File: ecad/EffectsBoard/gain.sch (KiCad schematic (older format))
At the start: 6 parts, among them Q1 2N4401BU

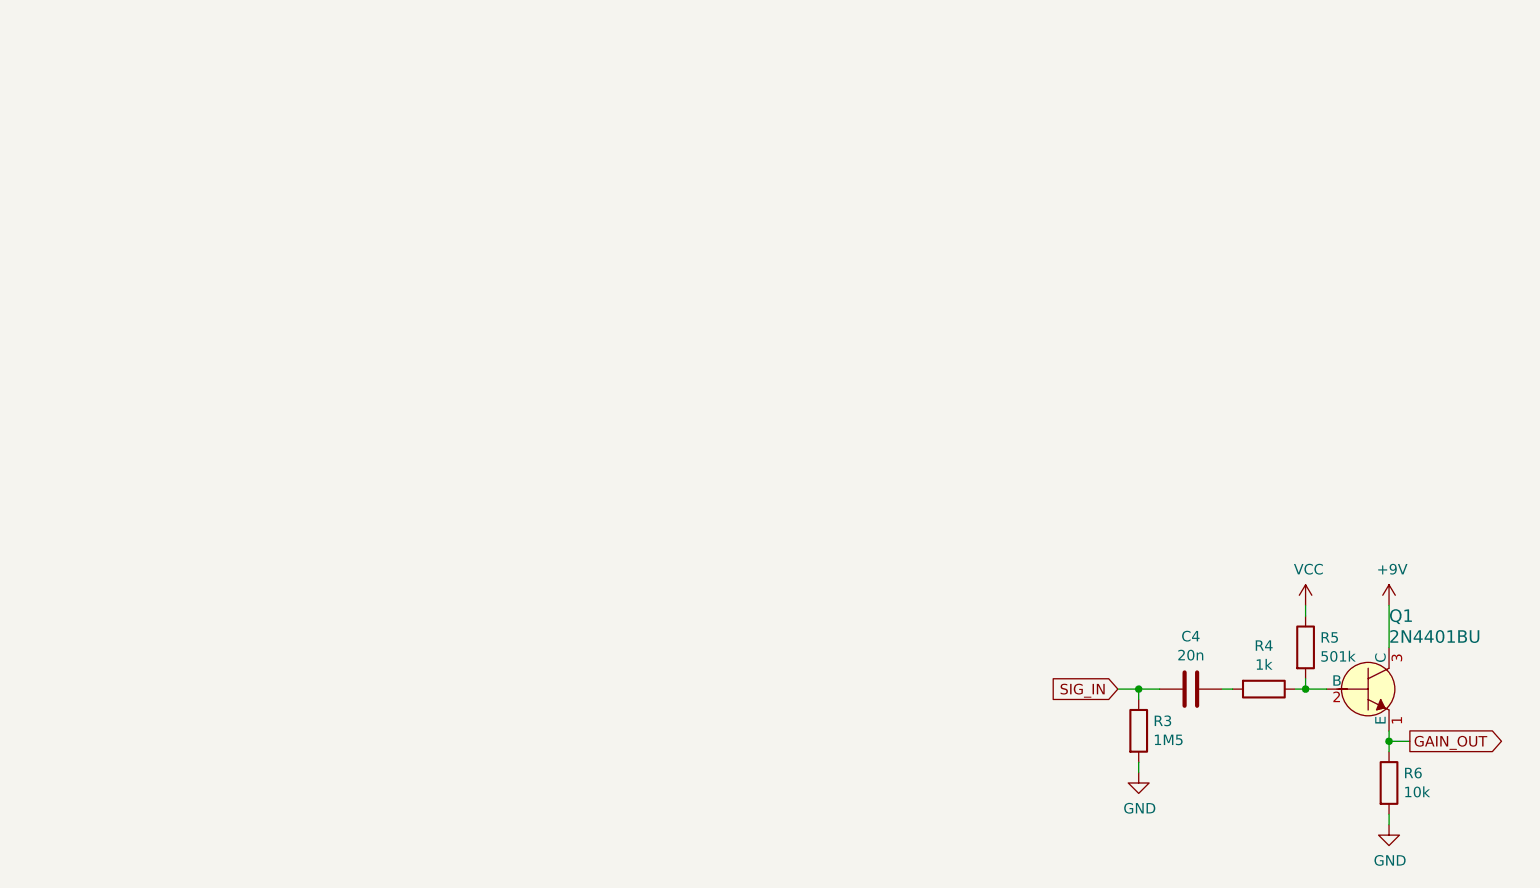
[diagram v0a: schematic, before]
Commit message: Rearrange schematics
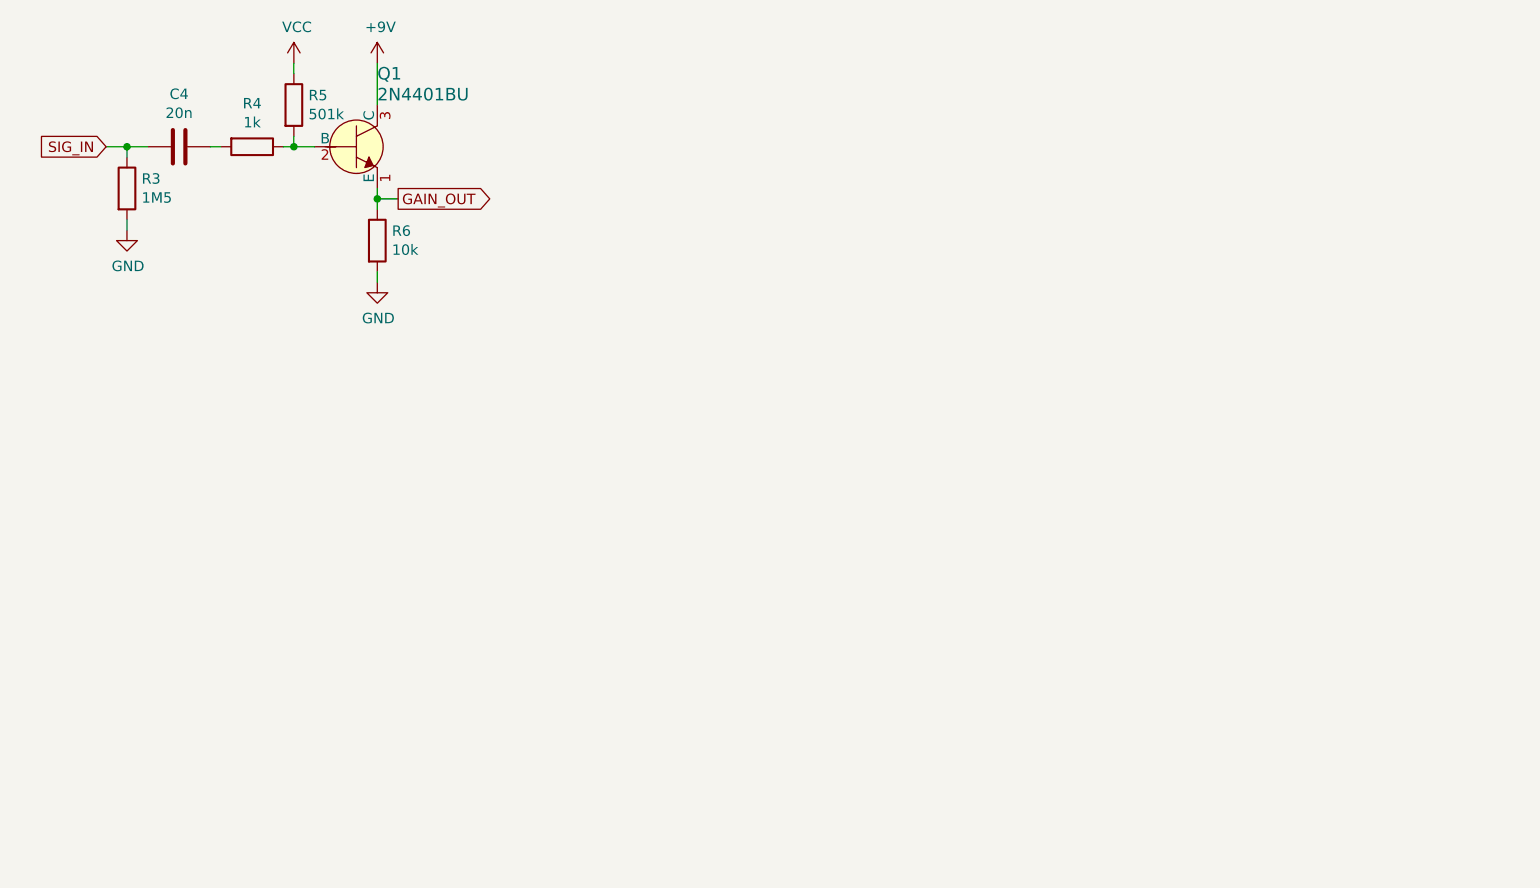
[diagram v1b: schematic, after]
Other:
- moved on the sheet: C4, Q1, R3, R4, R5, R6
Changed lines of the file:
@@
 L Device:R R?
 U 1 1 6030F08B
-P 5750 3900
+P 900 1300
 AR Path="/6030F08B" Ref="R?"  Part="1"
 AR Path="/60306390/6030F08B" Ref="R3"  Part="1"
-F 0 "R3" H 5820 3946 50  0000 L CNN
-F 1 "1M5" H 5820 3855 50  0000 L CNN
-F 2 "" V 5680 3900 50  0001 C CNN
-F 3 "~" H 5750 3900 50  0001 C CNN
-	1    5750 3900
+F 0 "R3" H 970 1346 50  0000 L CNN
+F 1 "1M5" H 970 1255 50  0000 L CNN
+F 2 "" V 830 1300 50  0001 C CNN
+F 3 "~" H 900 1300 50  0001 C CNN
+	1    900  1300
 	1    0    0    -1
 $EndComp
@@
 L power:GND #PWR?
 U 1 1 6030F091
-P 5750 4100
+P 900 1500
 AR Path="/6030F091" Ref="#PWR?"  Part="1"
 AR Path="/60306390/6030F091" Ref="#PWR0111"  Part="1"
-F 0 "#PWR0111" H 5750 3850 50  0001 C CNN
-F 1 "GND" H 5755 3927 50  0000 C CNN
-F 2 "" H 5750 4100 50  0001 C CNN
-F 3 "" H 5750 4100 50  0001 C CNN
-	1    5750 4100
+F 0 "#PWR0111" H 900 1250 50  0001 C CNN
+F 1 "GND" H 905 1327 50  0000 C CNN
+F 2 "" H 900 1500 50  0001 C CNN
+F 3 "" H 900 1500 50  0001 C CNN
+	1    900  1500
 	1    0    0    -1
 $EndComp
 Wire Wire Line
-	5750 4100 5750 4050
+	900  1500 900  1450
 Wire Wire Line
-	5750 3750 5750 3700
+	900  1150 900  1100
 Wire Wire Line
-	5750 3700 5650 3700
+	900  1100 800  1100
 $Comp
 L Device:C C?
 U 1 1 6030F09B
-P 6000 3700
+P 1150 1100
 AR Path="/6030F09B" Ref="C?"  Part="1"
 AR Path="/60306390/6030F09B" Ref="C4"  Part="1"
-F 0 "C4" V 5748 3700 50  0000 C CNN
-F 1 "20n" V 5839 3700 50  0000 C CNN
-F 2 "" H 6038 3550 50  0001 C CNN
-F 3 "~" H 6000 3700 50  0001 C CNN
-	1    6000 3700
+F 0 "C4" V 898 1100 50  0000 C CNN
+F 1 "20n" V 989 1100 50  0000 C CNN
+F 2 "" H 1188 950 50  0001 C CNN
+F 3 "~" H 1150 1100 50  0001 C CNN
+	1    1150 1100
 	0    1    1    0
 $EndComp
 Wire Wire Line
-	5850 3700 5750 3700
-Connection ~ 5750 3700
+	1000 1100 900  1100
+Connection ~ 900  1100
 $Comp
 L Device:R R?
 U 1 1 6030F0A3
-P 6350 3700
+P 1500 1100
 AR Path="/6030F0A3" Ref="R?"  Part="1"
 AR Path="/60306390/6030F0A3" Ref="R4"  Part="1"
-F 0 "R4" V 6143 3700 50  0000 C CNN
-F 1 "1k" V 6234 3700 50  0000 C CNN
-F 2 "" V 6280 3700 50  0001 C CNN
-F 3 "~" H 6350 3700 50  0001 C CNN
-	1    6350 3700
+F 0 "R4" V 1293 1100 50  0000 C CNN
+F 1 "1k" V 1384 1100 50  0000 C CNN
+F 2 "" V 1430 1100 50  0001 C CNN
+F 3 "~" H 1500 1100 50  0001 C CNN
+	1    1500 1100
 	0    1    1    0
 $EndComp
@@
 L Device:R R?
 U 1 1 6030F0A9
-P 6550 3500
+P 1700 900
 AR Path="/6030F0A9" Ref="R?"  Part="1"
 AR Path="/60306390/6030F0A9" Ref="R5"  Part="1"
-F 0 "R5" H 6620 3546 50  0000 L CNN
-F 1 "501k" H 6620 3455 50  0000 L CNN
-F 2 "" V 6480 3500 50  0001 C CNN
-F 3 "~" H 6550 3500 50  0001 C CNN
-	1    6550 3500
+F 0 "R5" H 1770 946 50  0000 L CNN
+F 1 "501k" H 1770 855 50  0000 L CNN
+F 2 "" V 1630 900 50  0001 C CNN
+F 3 "~" H 1700 900 50  0001 C CNN
+	1    1700 900
 	1    0    0    -1
 $EndComp
 Wire Wire Line
-	6150 3700 6200 3700
+	1300 1100 1350 1100
 Wire Wire Line
-	6550 3700 6550 3650
+	1700 1100 1700 1050
 Wire Wire Line
-	6500 3700 6550 3700
+	1650 1100 1700 1100
 Wire Wire Line
-	6550 3350 6550 3300
+	1700 750  1700 700
 $Comp
 L power:VCC #PWR?
 U 1 1 6030F0B3
-P 6550 3300
+P 1700 700
 AR Path="/6030F0B3" Ref="#PWR?"  Part="1"
 AR Path="/60306390/6030F0B3" Ref="#PWR0112"  Part="1"
-F 0 "#PWR0112" H 6550 3150 50  0001 C CNN
-F 1 "VCC" H 6565 3473 50  0000 C CNN
-F 2 "" H 6550 3300 50  0001 C CNN
-F 3 "" H 6550 3300 50  0001 C CNN
-	1    6550 3300
+F 0 "#PWR0112" H 1700 550 50  0001 C CNN
+F 1 "VCC" H 1715 873 50  0000 C CNN
+F 2 "" H 1700 700 50  0001 C CNN
+F 3 "" H 1700 700 50  0001 C CNN
+	1    1700 700
 	1    0    0    -1
 $EndComp
@@
 L dk_Transistors-Bipolar-BJT-Single:2N4401BU Q?
 U 1 1 6030F0C2
-P 6850 3700
+P 2000 1100
 AR Path="/6030F0C2" Ref="Q?"  Part="1"
 AR Path="/60306390/6030F0C2" Ref="Q1"  Part="1"
-F 0 "Q1" H 6950 4050 60  0000 L CNN
-F 1 "2N4401BU" H 6950 3950 60  0000 L CNN
-F 2 "digikey-footprints:TO-92-3" H 7050 3900 60  0001 L CNN
-F 3 "https://www.onsemi.com/pub/Collateral/MMBT4401-D.PDF" H 7050 4000 60  0001 L CNN
-F 4 "2N4401-ND" H 7050 4100 60  0001 L CNN "Digi-Key_PN"
-F 5 "2N4401BU" H 7050 4200 60  0001 L CNN "MPN"
-F 6 "Discrete Semiconductor Products" H 7050 4300 60  0001 L CNN "Category"
-F 7 "Transistors - Bipolar (BJT) - Single" H 7050 4400 60  0001 L CNN "Family"
-F 8 "https://www.onsemi.com/pub/Collateral/MMBT4401-D.PDF" H 7050 4500 60  0001 L CNN "DK_Datasheet_Link"
-F 9 "/product-detail/en/on-semiconductor/2N4401BU/2N4401-ND/1417" H 7050 4600 60  0001 L CNN "DK_Detail_Page"
-F 10 "TRANS NPN 40V 0.6A TO-92" H 7050 4700 60  0001 L CNN "Description"
-F 11 "ON Semiconductor" H 7050 4800 60  0001 L CNN "Manufacturer"
-F 12 "Active" H 7050 4900 60  0001 L CNN "Status"
-	1    6850 3700
+F 0 "Q1" H 2100 1450 60  0000 L CNN
+F 1 "2N4401BU" H 2100 1350 60  0000 L CNN
+F 2 "digikey-footprints:TO-92-3" H 2200 1300 60  0001 L CNN
+F 3 "https://www.onsemi.com/pub/Collateral/MMBT4401-D.PDF" H 2200 1400 60  0001 L CNN
+F 4 "2N4401-ND" H 2200 1500 60  0001 L CNN "Digi-Key_PN"
+F 5 "2N4401BU" H 2200 1600 60  0001 L CNN "MPN"
+F 6 "Discrete Semiconductor Products" H 2200 1700 60  0001 L CNN "Category"
+F 7 "Transistors - Bipolar (BJT) - Single" H 2200 1800 60  0001 L CNN "Family"
+F 8 "https://www.onsemi.com/pub/Collateral/MMBT4401-D.PDF" H 2200 1900 60  0001 L CNN "DK_Datasheet_Link"
+F 9 "/product-detail/en/on-semiconductor/2N4401BU/2N4401-ND/1417" H 2200 2000 60  0001 L CNN "DK_Detail_Page"
+F 10 "TRANS NPN 40V 0.6A TO-92" H 2200 2100 60  0001 L CNN "Description"
+F 11 "ON Semiconductor" H 2200 2200 60  0001 L CNN "Manufacturer"
+F 12 "Active" H 2200 2300 60  0001 L CNN "Status"
+	1    2000 1100
 	1    0    0    -1
 $EndComp
@@
 L power:+9V #PWR?
 U 1 1 6030F0C8
-P 6950 3300
+P 2100 700
 AR Path="/6030F0C8" Ref="#PWR?"  Part="1"
 AR Path="/60306390/6030F0C8" Ref="#PWR0113"  Part="1"
-F 0 "#PWR0113" H 6950 3150 50  0001 C CNN
-F 1 "+9V" H 6965 3473 50  0000 C CNN
-F 2 "" H 6950 3300 50  0001 C CNN
-F 3 "" H 6950 3300 50  0001 C CNN
-	1    6950 3300
+F 0 "#PWR0113" H 2100 550 50  0001 C CNN
+F 1 "+9V" H 2115 873 50  0000 C CNN
+F 2 "" H 2100 700 50  0001 C CNN
+F 3 "" H 2100 700 50  0001 C CNN
+	1    2100 700
 	1    0    0    -1
 $EndComp
 Wire Wire Line
-	6950 3300 6950 3500
+	2100 700  2100 900
 Wire Wire Line
-	6650 3700 6550 3700
-Connection ~ 6550 3700
+	1800 1100 1700 1100
+Connection ~ 1700 1100
 $Comp
 L Device:R R?
 U 1 1 6030F0D1
-P 6950 4150
+P 2100 1550
 AR Path="/6030F0D1" Ref="R?"  Part="1"
 AR Path="/60306390/6030F0D1" Ref="R6"  Part="1"
-F 0 "R6" H 7020 4196 50  0000 L CNN
-F 1 "10k" H 7020 4105 50  0000 L CNN
-F 2 "" V 6880 4150 50  0001 C CNN
-F 3 "~" H 6950 4150 50  0001 C CNN
-	1    6950 4150
+F 0 "R6" H 2170 1596 50  0000 L CNN
+F 1 "10k" H 2170 1505 50  0000 L CNN
+F 2 "" V 2030 1550 50  0001 C CNN
+F 3 "~" H 2100 1550 50  0001 C CNN
+	1    2100 1550
 	1    0    0    -1
 $EndComp
@@
 L power:GND #PWR?
 U 1 1 6030F0D7
-P 6950 4350
+P 2100 1750
 AR Path="/6030F0D7" Ref="#PWR?"  Part="1"
 AR Path="/60306390/6030F0D7" Ref="#PWR0114"  Part="1"
-F 0 "#PWR0114" H 6950 4100 50  0001 C CNN
-F 1 "GND" H 6955 4177 50  0000 C CNN
-F 2 "" H 6950 4350 50  0001 C CNN
-F 3 "" H 6950 4350 50  0001 C CNN
-	1    6950 4350
+F 0 "#PWR0114" H 2100 1500 50  0001 C CNN
+F 1 "GND" H 2105 1577 50  0000 C CNN
+F 2 "" H 2100 1750 50  0001 C CNN
+F 3 "" H 2100 1750 50  0001 C CNN
+	1    2100 1750
 	1    0    0    -1
 $EndComp
 Wire Wire Line
-	6950 4350 6950 4300
-Text GLabel 5650 3700 0    50   Input ~ 0
+	2100 1750 2100 1700
+Text GLabel 800  1100 0    50   Input ~ 0
 SIG_IN
-Text GLabel 7050 3950 2    50   Output ~ 0
+Text GLabel 2200 1350 2    50   Output ~ 0
 GAIN_OUT
 Wire Wire Line
-	6950 3900 6950 3950
+	2100 1300 2100 1350
 Wire Wire Line
-	6950 3950 7050 3950
-Connection ~ 6950 3950
+	2100 1350 2200 1350
+Connection ~ 2100 1350
 Wire Wire Line
-	6950 3950 6950 4000
+	2100 1350 2100 1400
 $EndSCHEMATC

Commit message: Update ecad autosave
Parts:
- C4: footprint (none) -> Capacitor_SMD:C_0805_2012Metric_Pad1.18x1.45mm_HandSolder
- R3, R4, R5, R6: footprint (none) -> Resistor_SMD:R_0805_2012Metric_Pad1.20x1.40mm_HandSolder
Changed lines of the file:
@@
 F 0 "R3" H 970 1346 50  0000 L CNN
 F 1 "1M5" H 970 1255 50  0000 L CNN
-F 2 "" V 830 1300 50  0001 C CNN
+F 2 "Resistor_SMD:R_0805_2012Metric_Pad1.20x1.40mm_HandSolder" V 830 1300 50  0001 C CNN
 F 3 "~" H 900 1300 50  0001 C CNN
 	1    900  1300
@@
 F 0 "C4" V 898 1100 50  0000 C CNN
 F 1 "20n" V 989 1100 50  0000 C CNN
-F 2 "" H 1188 950 50  0001 C CNN
+F 2 "Capacitor_SMD:C_0805_2012Metric_Pad1.18x1.45mm_HandSolder" H 1188 950 50  0001 C CNN
 F 3 "~" H 1150 1100 50  0001 C CNN
 	1    1150 1100
@@
 F 0 "R4" V 1293 1100 50  0000 C CNN
 F 1 "1k" V 1384 1100 50  0000 C CNN
-F 2 "" V 1430 1100 50  0001 C CNN
+F 2 "Resistor_SMD:R_0805_2012Metric_Pad1.20x1.40mm_HandSolder" V 1430 1100 50  0001 C CNN
 F 3 "~" H 1500 1100 50  0001 C CNN
 	1    1500 1100
@@
 F 0 "R5" H 1770 946 50  0000 L CNN
 F 1 "501k" H 1770 855 50  0000 L CNN
-F 2 "" V 1630 900 50  0001 C CNN
+F 2 "Resistor_SMD:R_0805_2012Metric_Pad1.20x1.40mm_HandSolder" V 1630 900 50  0001 C CNN
 F 3 "~" H 1700 900 50  0001 C CNN
 	1    1700 900
@@
 F 0 "R6" H 2170 1596 50  0000 L CNN
 F 1 "10k" H 2170 1505 50  0000 L CNN
-F 2 "" V 2030 1550 50  0001 C CNN
+F 2 "Resistor_SMD:R_0805_2012Metric_Pad1.20x1.40mm_HandSolder" V 2030 1550 50  0001 C CNN
 F 3 "~" H 2100 1550 50  0001 C CNN
 	1    2100 1550
